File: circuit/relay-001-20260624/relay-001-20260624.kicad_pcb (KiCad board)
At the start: 2 copper layers, 169 x 126.3 mm, 15 parts, among them J1 Conn_01x03_Pin, J10 Conn_01x02_Pin, J11 Conn_01x02_Pin, J12 Conn_01x02_Pin, J13 Conn_01x02_Pin, J14 Conn_01x02_Pin, J15 Conn_01x02_Pin, J2 Conn_02x05_Odd_Even, J3 Conn_02x08_Odd_Even, J4 Conn_02x09_Odd_Even, J5 Conn_01x02_Pin, J6 Conn_01x02_Pin, J7 Conn_01x02_Pin, J8 Conn_01x02_Pin, J9 Conn_01x02_Pin

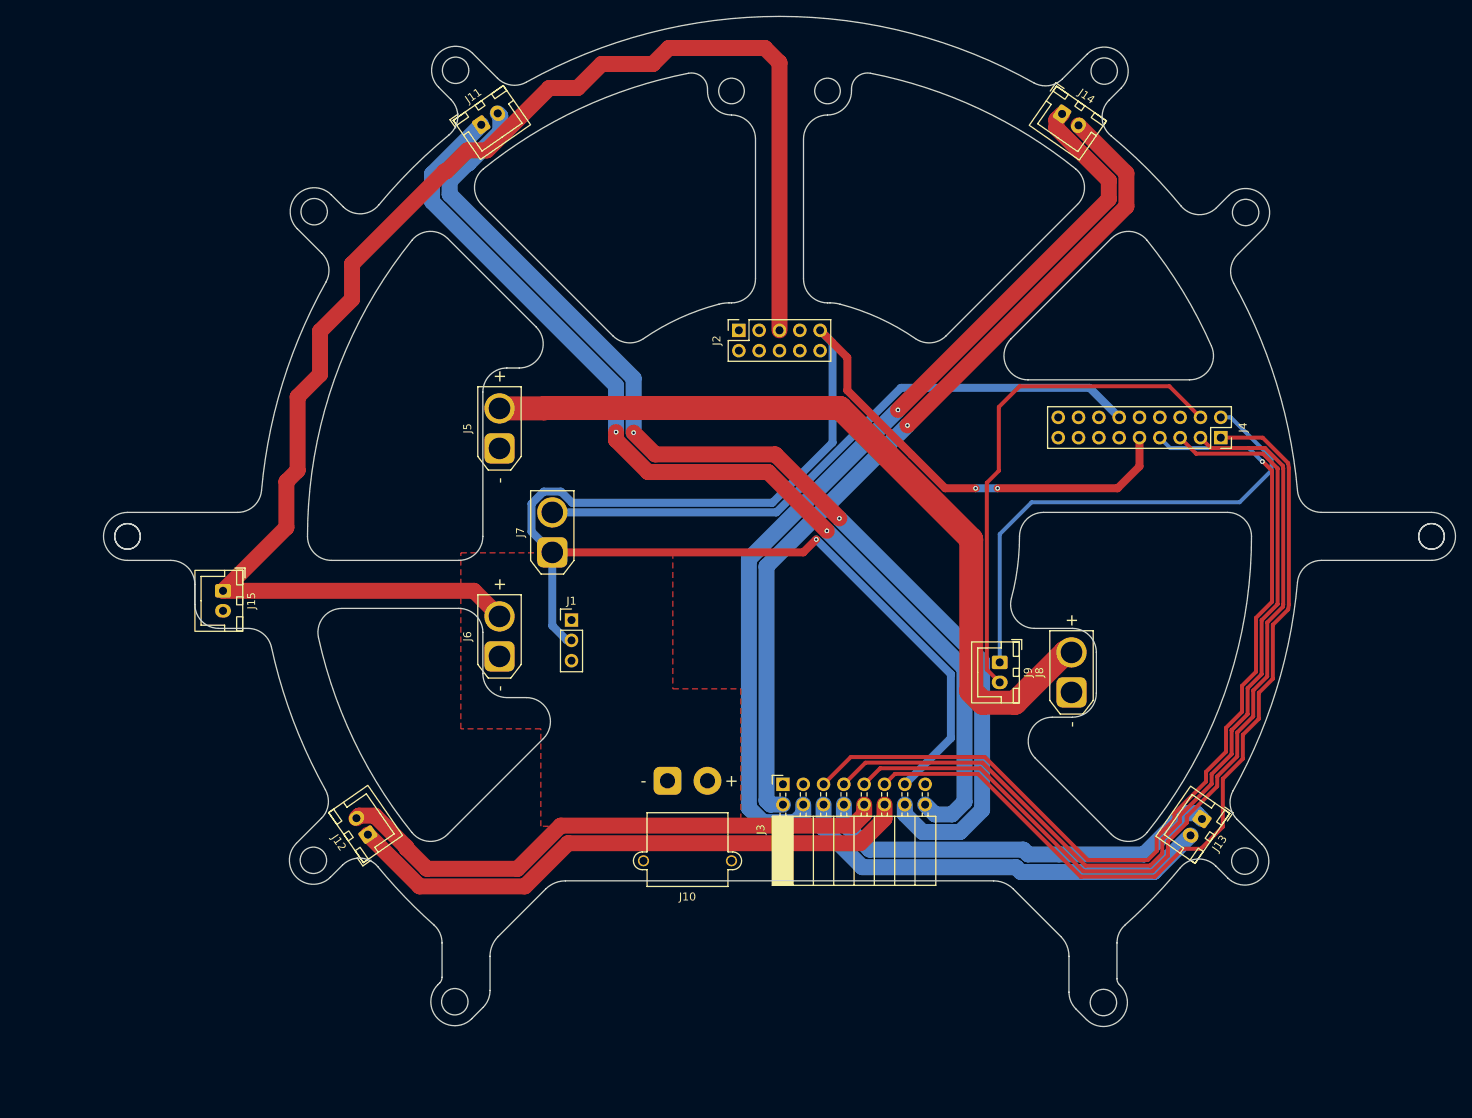
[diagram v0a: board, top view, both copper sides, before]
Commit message: Update 供給基板のボード図を更新
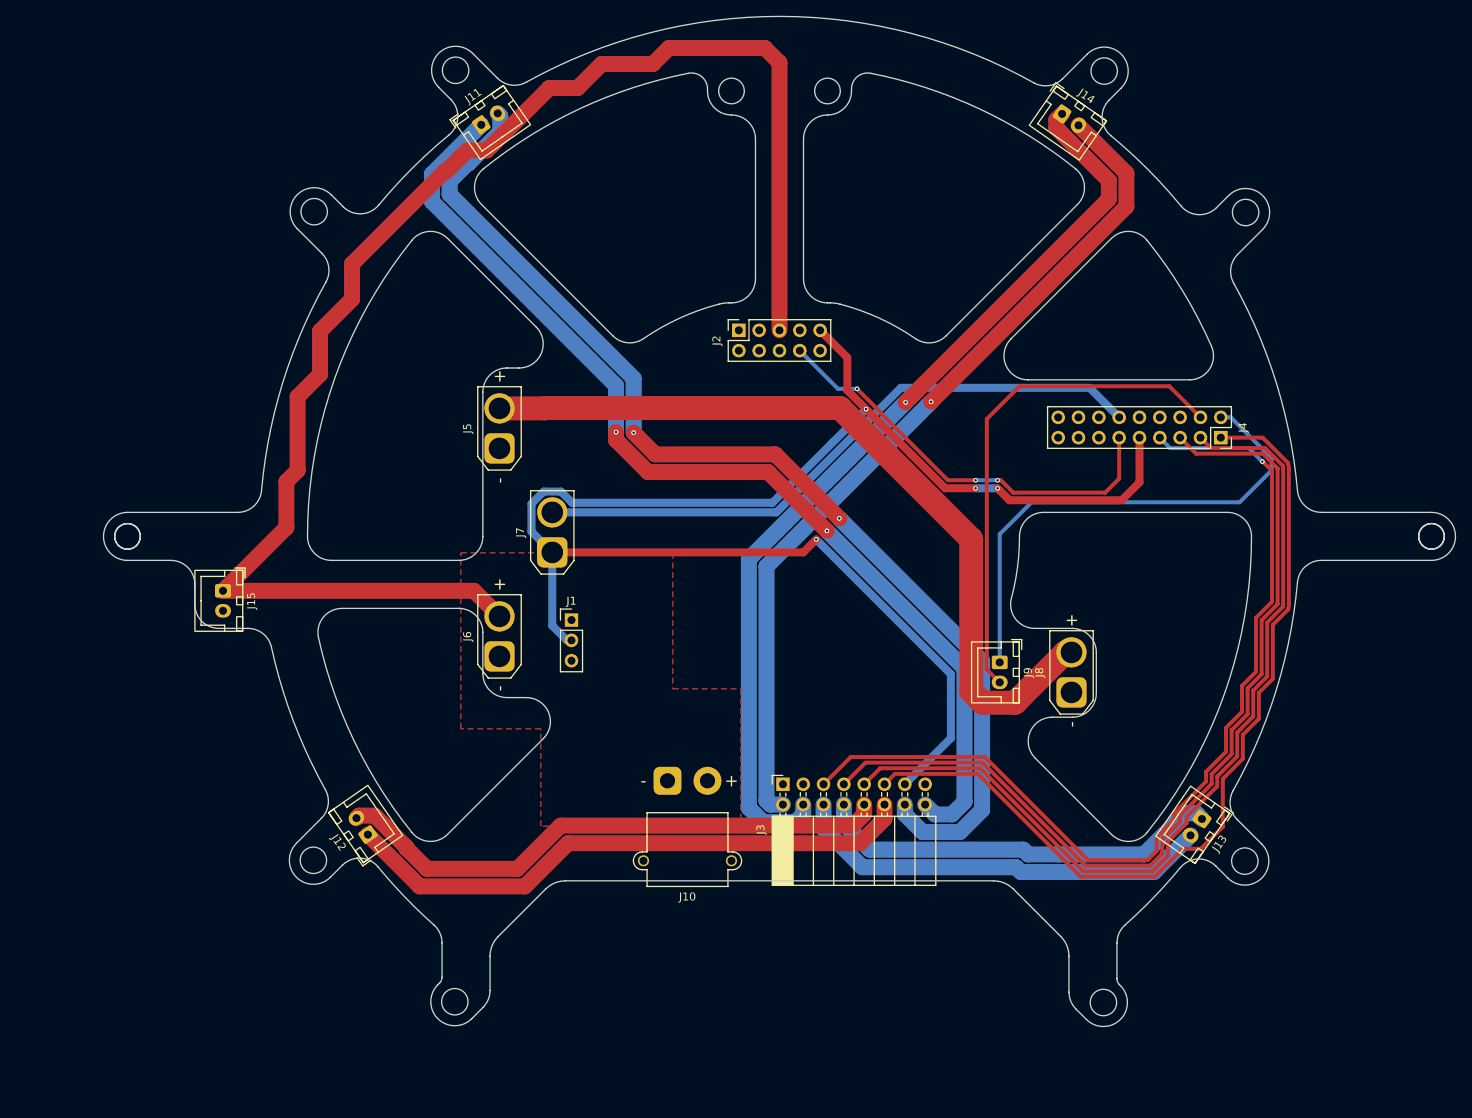
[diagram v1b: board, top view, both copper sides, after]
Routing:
- net BallCatch_{Front}: track 0.00 -> 53.2 mm, vias 0 -> 3
- net +3.3V: track 205.0 -> 198.6 mm, vias 3 -> 4

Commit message: Update 供給基板のボード図を更新
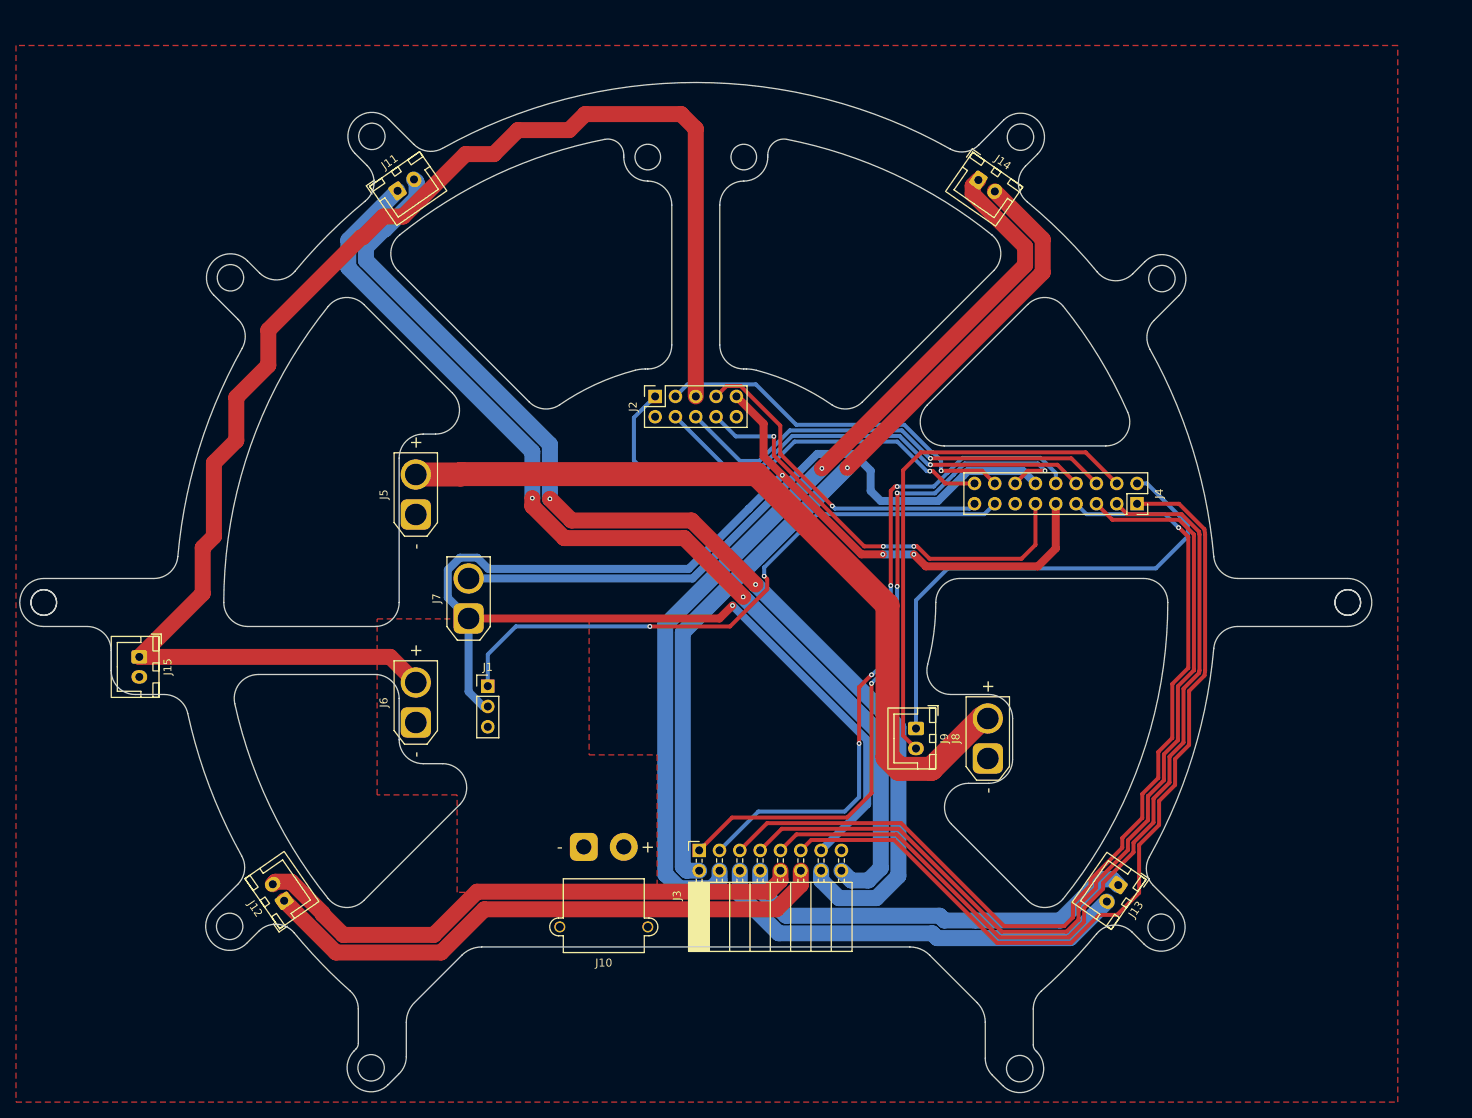
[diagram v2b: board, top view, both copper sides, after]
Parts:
- moved J8 13.3 mm to (172.3, 114.5)
- moved J7 13.3 mm to (107.4, 97.0)
- moved J11 13.3 mm to (98.5, 43.6)
- moved J1 13.3 mm to (109.8, 105.5)
- moved J10 13.3 mm to (121.8, 125.6)
- moved J12 13.3 mm to (84.3, 132.3)
- moved J3 13.3 mm to (136.2, 126.0)
- moved J4 13.3 mm to (190.9, 82.7)
- moved J5 13.3 mm to (100.8, 84.0)
- moved J6 13.3 mm to (100.8, 110.0)
- moved J9 13.3 mm to (163.3, 110.8)
- moved J14 13.3 mm to (171.1, 42.2)
- moved J2 13.3 mm to (130.7, 69.3)
- moved J15 13.3 mm to (66.2, 101.8)
- moved J13 13.3 mm to (188.6, 130.4)
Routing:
- net BallCatch_{Back}: track 0.00 -> 88.2 mm, vias 0 -> 4
- net Motor4_{PWM}: track 0.00 -> 84.7 mm, vias 0 -> 4
- net Dribbler_{Back}: track 0.00 -> 77.3 mm, vias 0 -> 2
- net EN_{Dribbler-Front}: track 0.00 -> 56.7 mm, vias 0 -> 1
- net PH_{Dribbler-Front}: track 0.00 -> 56.7 mm, vias 0 -> 1
- net EN_{Boost}: track 0.00 -> 56.0 mm, vias 0 -> 1
- net Kick_{Chip}: track 0.00 -> 46.4 mm, vias 0 -> 1
- net Kick_{Stroke}: track 0.00 -> 41.5 mm, vias 0 -> 1
- net +5V: track 78.8 -> 83.4 mm
- net BallCatch_{Front}: track 53.2 -> 54.6 mm
- net RX_{teensy}-TX_{Arduino}-5V: track 63.6 -> 64.7 mm
- added copper zone on F.Cu, net GND
